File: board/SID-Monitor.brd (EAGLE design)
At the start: 69.8 x 120.7 mm, 107 parts, among them IC1 LM317, IC2 LM337, IC3 TLE2082, IC4 TLE2082, IC5 MAX275ACP, IC6 TLE2082, IC7 TLE2082, IC8 TLE2082, IC9 PHOTON_WITH_HEADERS, J101 POWERJACK-PTH, Q201 2N2222, Q202 2N2222, X201 5414373, X301 5414373

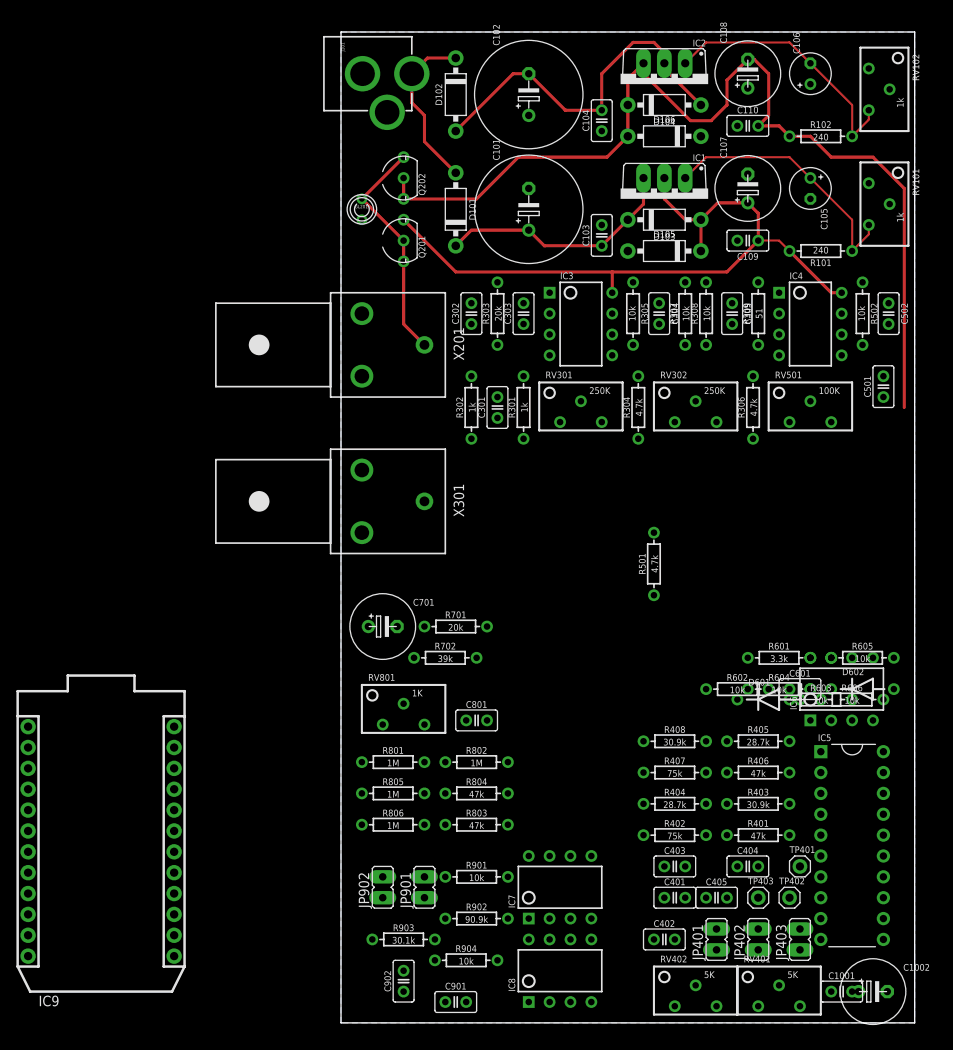
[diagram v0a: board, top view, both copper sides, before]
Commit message: Board layout first pass
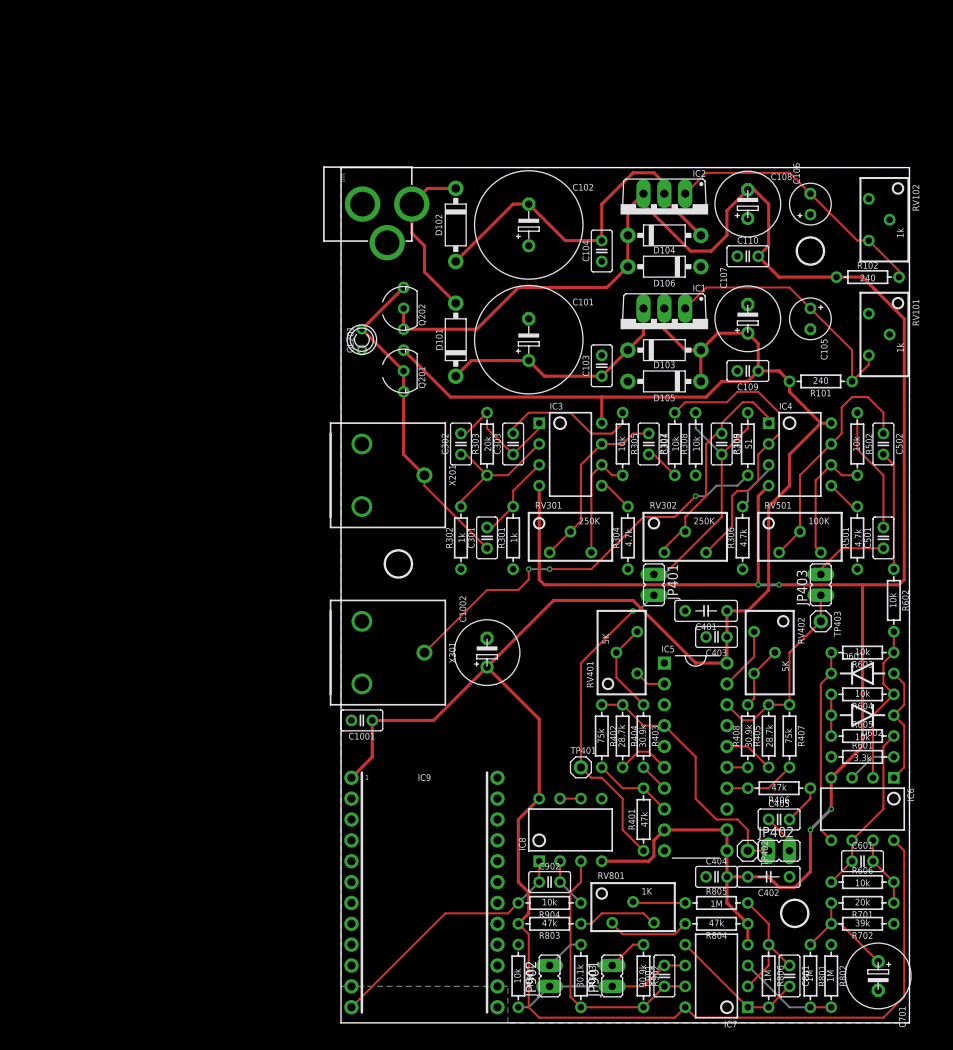
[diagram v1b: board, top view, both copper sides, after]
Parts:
- added U$1, U$2, U$3: (no value), SaintGimp:MOUNTING-HOLE-3.2MM
- C401, C402: device SaintGimp:CAPACITOR-2.5MM -> SaintGimp:CAPACITOR-5MM
- IC9: value PHOTON_WITH_HEADERS -> PHOTON
- moved C701 73.8 mm to (65.4, 5.71), turned to 270 degrees
- moved C1001 67.1 mm to (2.54, 36.8), turned to 180 degrees
- moved C1002 62.5 mm to (17.8, 45.1), turned to 90 degrees
- moved R702 60.2 mm to (63.5, 12.1), turned to 180 degrees
- moved R701 59.9 mm to (63.5, 14.6), turned to 180 degrees
- moved R801 57.1 mm to (57.1, 5.71), turned to 270 degrees
- moved IC9 51.0 mm to (10.2, 15.9)
- moved R802 50.4 mm to (59.7, 5.71), turned to 270 degrees
- moved R806 49.3 mm to (52.1, 5.71), turned to 270 degrees
- moved C801 49.2 mm to (54.6, 5.71), turned to 270 degrees
- moved RV401 45.5 mm to (34.3, 45.1), turned to 90 degrees
- moved JP401 43.8 mm to (38.1, 53.3), turned to 180 degrees
- moved JP403 43.3 mm to (58.4, 53.3)
- moved RV402 42.2 mm to (52.1, 45.1), turned to 270 degrees
- moved R805 41.6 mm to (45.7, 14.6)
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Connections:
- new net N$39: IC8.6, IC8.7
- net GND: now also IC8.5
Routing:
- net +5V: track 86.3 -> 296.3 mm
- net -5V: track 121.6 -> 278.1 mm, vias 0 -> 4
- net N$38: track 0.00 -> 49.1 mm, vias 0 -> 3
- net N$20: track 0.00 -> 39.1 mm, vias 0 -> 1
- net N$15: track 0.00 -> 36.2 mm
- net N$55: track 0.00 -> 32.6 mm
- net N$18: track 0.00 -> 32.1 mm
- net N$59: track 0.00 -> 31.7 mm
- net N$11: track 0.00 -> 31.6 mm
- net N$35: track 0.00 -> 29.7 mm
- net N$17: track 0.00 -> 27.7 mm
- net N$28: track 0.00 -> 24.1 mm
- net N$45: track 0.00 -> 23.9 mm
- net N$58: track 0.00 -> 22.4 mm
- net N$13: track 0.00 -> 22.1 mm
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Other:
- board size 69.8 x 120.7 mm -> 69.2 x 104.1 mm
